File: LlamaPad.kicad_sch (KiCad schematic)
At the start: 0 parts

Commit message: feat: finish schematic rev1
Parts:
- added A1: RaspberryPi_Pico, Module:RaspberryPi_Pico_Common_Unspecified, symbol MCU_Module:RaspberryPi_Pico
- added D1, D10, D11, D12, D13, D14, D15, D16, D17, D18, D2, D3, D4, D5, D6, D7, D8, D9: D, Diode_THT:D_DO-35_SOD27_P7.62mm_Horizontal, symbol Device:D
- added D19, D20, D21, D22, D23, D24, D25, D26, D27, D28, D29, D30, D31, D32, D33, D34: SK6812MINI-E, HackPad:SK6812MINI-E_fixed, symbol SK6812MINI-E:SK6812MINI-E
- added J1: Conn_01x04_Pin, Connector_PinHeader_1.27mm:PinHeader_1x04_P1.27mm_Vertical, symbol Connector:Conn_01x04_Pin
- added REC_A1, REC_B1: RotaryEncoder_Switch, HackPad:RotaryEncoder_Alps_EC11E-Switch_Vertical_H20mm, symbol Device:RotaryEncoder_Switch
- added SW1, SW10, SW11, SW12, SW13, SW14, SW15, SW16, SW2, SW3, SW4, SW5, SW6, SW7, SW8, SW9: SW_Push, Button_Switch_Keyboard:SW_Cherry_MX_1.00u_PCB, symbol Switch:SW_Push
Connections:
- new net: D9.2 (A), SW9.2
- new net: D21.2 (DOUT), D25.4 (DIN)
- new net: D21.4 (DIN), D32.2 (DOUT)
- new net: D15.2 (A), SW14.2
- new net: D4.2 (A), SW4.2
- new net: D30.2 (DOUT), D34.4 (DIN)
- new net: D19.2 (DOUT), D23.4 (DIN)
- new net: D28.2 (DOUT), D32.4 (DIN)
- new net: D26.2 (DOUT), D30.4 (DIN)
- new net: D22.2 (DOUT), D26.4 (DIN)
- new net: D12.2 (A), SW12.2
- new net: D14.2 (A), SW15.2
- new net: D8.2 (A), SW8.2
- new net: D27.2 (DOUT), D31.4 (DIN)
- new net: D23.2 (DOUT), D27.4 (DIN)
- new net: D24.2 (DOUT), D28.4 (DIN)
- new net: D22.4 (DIN), D33.2 (DOUT)
- new net: D10.2 (A), SW10.2
- new net: D29.2 (DOUT), D33.4 (DIN)
- new net: D1.2 (A), SW1.2
- new net: D6.2 (A), SW6.2
- new net: D5.2 (A), SW5.2
- new net: D20.2 (DOUT), D24.4 (DIN)
- new net: D25.2 (DOUT), D29.4 (DIN)
- new net: D11.2 (A), SW11.2
- new net: D20.4 (DIN), D31.2 (DOUT)
- new net: D7.2 (A), SW7.2
- new net: D3.2 (A), SW3.2
- new net: D16.2 (A), SW13.2
- new net: D2.2 (A), SW2.2
- new net: D13.2 (A), SW16.2
- new net ARGB_DATA: A1.17 (GPIO13), D19.4 (DIN)
- new net COL0: A1.6 (GPIO4), SW1.1, SW2.1, SW3.1, SW4.1
- new net COL1: A1.7 (GPIO5), SW5.1, SW6.1, SW7.1, SW8.1
- new net COL2: A1.9 (GPIO6), SW10.1, SW11.1, SW12.1, SW9.1
- new net COL3: A1.10 (GPIO7), SW13.1, SW14.1, SW15.1, SW16.1
- new net COL4: A1.11 (GPIO8), REC_A1.S2, REC_B1.S2
- new net GND: A1.13 (GND), A1.18 (GND), A1.23 (GND), A1.28 (GND), A1.3 (GND), A1.38 (GND), A1.8 (GND), D19.3 (VSS), D20.3 (VSS), D21.3 (VSS), D22.3 (VSS), D23.3 (VSS), D24.3 (VSS), D25.3 (VSS), D26.3 (VSS), D27.3 (VSS), D28.3 (VSS), D29.3 (VSS), D30.3 (VSS), D31.3 (VSS), D32.3 (VSS), D33.3 (VSS), D34.3 (VSS), J1.4 (Pin_4), REC_A1.C, REC_B1.C
- new net OLED_SCL: A1.20 (GPIO15), J1.2 (Pin_2)
- new net OLED_SDA: A1.19 (GPIO14), J1.1 (Pin_1)
- new net REC_A1: A1.12 (GPIO9), REC_A1.B
- new net REC_A2: A1.14 (GPIO10), REC_A1.A
- new net REC_B1: A1.15 (GPIO11), REC_B1.B
- new net REC_B2: A1.16 (GPIO12), REC_B1.A
- new net REC_SW_A2: D18.2 (A), REC_A1.S1
- new net REC_SW_B2: D17.2 (A), REC_B1.S1
- new net ROW0: A1.1 (GPIO0), D1.1 (K), D16.1 (K), D17.1 (K), D5.1 (K), D9.1 (K)
- new net ROW1: A1.2 (GPIO1), D10.1 (K), D15.1 (K), D18.1 (K), D2.1 (K), D6.1 (K)
- new net ROW2: A1.4 (GPIO2), D11.1 (K), D14.1 (K), D3.1 (K), D7.1 (K)
- new net ROW3: A1.5 (GPIO3), D12.1 (K), D13.1 (K), D4.1 (K), D8.1 (K)
- new net VCC: A1.40 (VBUS), D19.1 (VDD), D20.1 (VDD), D21.1 (VDD), D22.1 (VDD), D23.1 (VDD), D24.1 (VDD), D25.1 (VDD), D26.1 (VDD), D27.1 (VDD), D28.1 (VDD), D29.1 (VDD), D30.1 (VDD), D31.1 (VDD), D32.1 (VDD), D33.1 (VDD), D34.1 (VDD), J1.3 (Pin_3)
- no-connect marks 0 -> 17
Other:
- note added: "OLED DISPLAY"
- note added: "PICO"
- note added: "ROTARY ENCODER"
- note added: "SWITCH ARGB"
- note added: "SWITCH MATRIX"

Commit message: feat: PCB rev1 (no traces)
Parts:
- J1: footprint Connector_PinHeader_1.27mm:PinHeader_1x04_P1.27mm_Vertical -> Connector_PinHeader_2.54mm:PinHeader_1x04_P2.54mm_Vertical
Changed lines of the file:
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@@
 			)
 		)
-		(property "Footprint" "Connector_PinHeader_1.27mm:PinHeader_1x04_P1.27mm_Vertical"
+		(property "Footprint" "Connector_PinHeader_2.54mm:PinHeader_1x04_P2.54mm_Vertical"
 			(at 229.87 130.81 0)
 			(effects

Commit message: feat: footprint stuff
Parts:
- SW1, SW10, SW11, SW12, SW13, SW14, SW15, SW16, SW2, SW3, SW4, SW5, SW6, SW7, SW8, SW9: footprint Button_Switch_Keyboard:SW_Cherry_MX_1.00u_PCB -> MX_Hotswap:MX-Hotswap-1U
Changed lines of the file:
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@@
 			)
 		)
-		(property "Footprint" "Button_Switch_Keyboard:SW_Cherry_MX_1.00u_PCB"
+		(property "Footprint" "MX_Hotswap:MX-Hotswap-1U"
 			(at 95.25 57.15 0)
 			(effects
@@
 			)
 		)
-		(property "Footprint" "Button_Switch_Keyboard:SW_Cherry_MX_1.00u_PCB"
+		(property "Footprint" "MX_Hotswap:MX-Hotswap-1U"
 			(at 95.25 69.85 0)
 			(effects
@@
 			)
 		)
-		(property "Footprint" "Button_Switch_Keyboard:SW_Cherry_MX_1.00u_PCB"
+		(property "Footprint" "MX_Hotswap:MX-Hotswap-1U"
 			(at 59.69 82.55 0)
 			(effects
@@
 			)
 		)
-		(property "Footprint" "Button_Switch_Keyboard:SW_Cherry_MX_1.00u_PCB"
+		(property "Footprint" "MX_Hotswap:MX-Hotswap-1U"
 			(at 41.91 44.45 0)
 			(effects
@@
 			)
 		)
-		(property "Footprint" "Button_Switch_Keyboard:SW_Cherry_MX_1.00u_PCB"
+		(property "Footprint" "MX_Hotswap:MX-Hotswap-1U"
 			(at 59.69 57.15 0)
 			(effects
@@
 			)
 		)
-		(property "Footprint" "Button_Switch_Keyboard:SW_Cherry_MX_1.00u_PCB"
+		(property "Footprint" "MX_Hotswap:MX-Hotswap-1U"
 			(at 59.69 44.45 0)
 			(effects
@@
 			)
 		)
-		(property "Footprint" "Button_Switch_Keyboard:SW_Cherry_MX_1.00u_PCB"
+		(property "Footprint" "MX_Hotswap:MX-Hotswap-1U"
 			(at 77.47 69.85 0)
 			(effects
@@
 			)
 		)
-		(property "Footprint" "Button_Switch_Keyboard:SW_Cherry_MX_1.00u_PCB"
+		(property "Footprint" "MX_Hotswap:MX-Hotswap-1U"
 			(at 77.47 82.55 0)
 			(effects
@@
 			)
 		)
-		(property "Footprint" "Button_Switch_Keyboard:SW_Cherry_MX_1.00u_PCB"
+		(property "Footprint" "MX_Hotswap:MX-Hotswap-1U"
 			(at 41.91 82.55 0)
 			(effects
@@
 			)
 		)
-		(property "Footprint" "Button_Switch_Keyboard:SW_Cherry_MX_1.00u_PCB"
+		(property "Footprint" "MX_Hotswap:MX-Hotswap-1U"
 			(at 77.47 57.15 0)
 			(effects
@@
 			)
 		)
-		(property "Footprint" "Button_Switch_Keyboard:SW_Cherry_MX_1.00u_PCB"
+		(property "Footprint" "MX_Hotswap:MX-Hotswap-1U"
 			(at 41.91 57.15 0)
 			(effects
@@
 			)
 		)
-		(property "Footprint" "Button_Switch_Keyboard:SW_Cherry_MX_1.00u_PCB"
+		(property "Footprint" "MX_Hotswap:MX-Hotswap-1U"
 			(at 59.69 69.85 0)
 			(effects
@@
 			)
 		)
-		(property "Footprint" "Button_Switch_Keyboard:SW_Cherry_MX_1.00u_PCB"
+		(property "Footprint" "MX_Hotswap:MX-Hotswap-1U"
 			(at 77.47 44.45 0)
 			(effects
@@
 			)
 		)
-		(property "Footprint" "Button_Switch_Keyboard:SW_Cherry_MX_1.00u_PCB"
+		(property "Footprint" "MX_Hotswap:MX-Hotswap-1U"
 			(at 41.91 69.85 0)
 			(effects
@@
 			)
 		)
-		(property "Footprint" "Button_Switch_Keyboard:SW_Cherry_MX_1.00u_PCB"
+		(property "Footprint" "MX_Hotswap:MX-Hotswap-1U"
 			(at 95.25 82.55 0)
 			(effects
@@
 			)
 		)
-		(property "Footprint" "Button_Switch_Keyboard:SW_Cherry_MX_1.00u_PCB"
+		(property "Footprint" "MX_Hotswap:MX-Hotswap-1U"
 			(at 95.25 44.45 0)
 			(effects

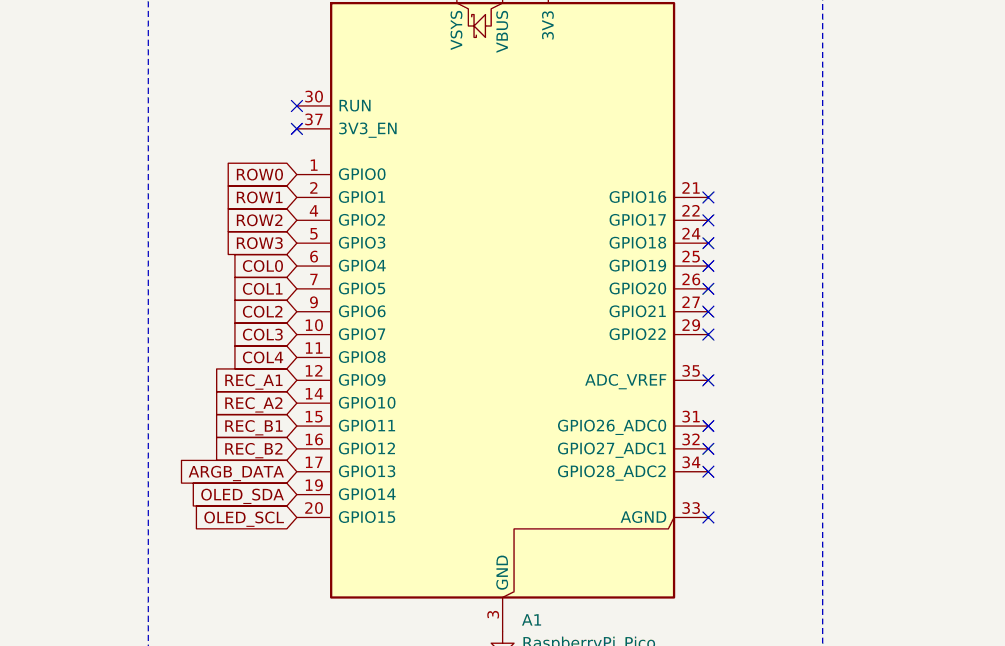
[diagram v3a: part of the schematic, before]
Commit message: feat: route the pcb and change schematic to be easier
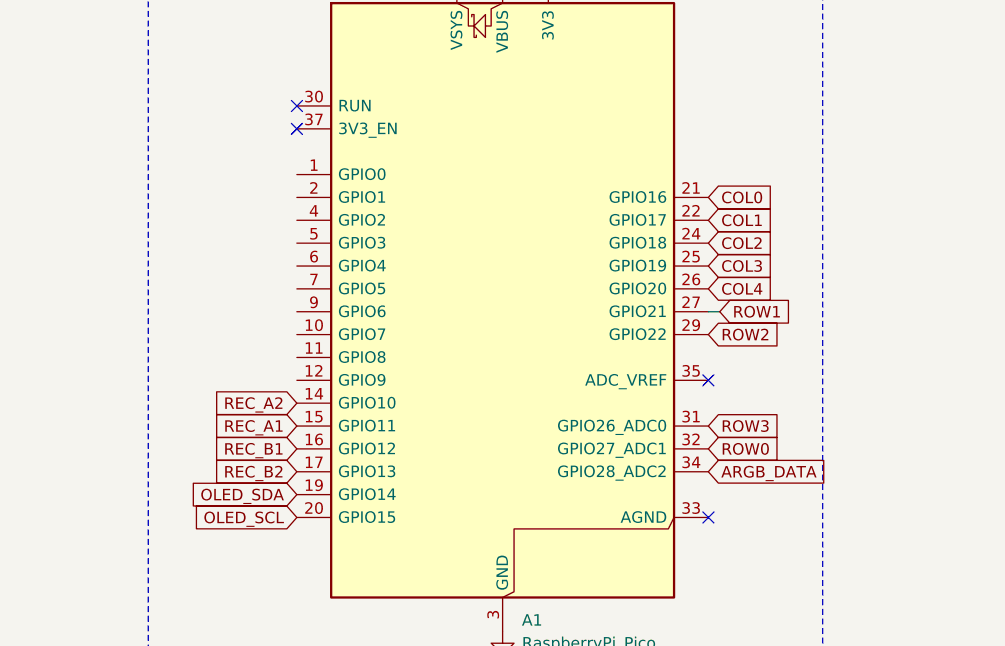
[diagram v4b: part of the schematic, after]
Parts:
- D19, D20, D21, D22, D23, D24, D25, D26, D27, D28, D29, D30, D31, D32, D33, D34: footprint HackPad:SK6812MINI-E_fixed -> Llama_Other:SK6812MINI-E_fixed
- REC_A1, REC_B1: footprint HackPad:RotaryEncoder_Alps_EC11E-Switch_Vertical_H20mm -> RotaryEncoder:RotaryEncoder_Alps_EC11E-Switch_Vertical_H20mm
- SW1, SW10, SW11, SW12, SW13, SW14, SW15, SW16, SW2, SW3, SW4, SW5, SW6, SW7, SW8, SW9: footprint MX_Hotswap:MX-Hotswap-1U -> Switch_MX_Hotswap:MX-Hotswap-1U
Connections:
- net ARGB_DATA: now also A1.34 (GPIO28_ADC2); no longer A1.17 (GPIO13)
- net COL0: now also A1.21 (GPIO16); no longer A1.6 (GPIO4)
- net COL1: now also A1.22 (GPIO17); no longer A1.7 (GPIO5)
- net COL2: now also A1.24 (GPIO18); no longer A1.9 (GPIO6)
- net COL3: now also A1.25 (GPIO19); no longer A1.10 (GPIO7)
- net COL4: now also A1.26 (GPIO20); no longer A1.11 (GPIO8)
- net REC_A1: now also A1.15 (GPIO11); no longer A1.12 (GPIO9)
- net REC_B1: now also A1.16 (GPIO12); no longer A1.15 (GPIO11)
- net REC_B2: now also A1.17 (GPIO13); no longer A1.16 (GPIO12)
- net ROW0: now also A1.32 (GPIO27_ADC1); no longer A1.1 (GPIO0)
- net ROW1: now also A1.27 (GPIO21); no longer A1.2 (GPIO1)
- net ROW2: now also A1.29 (GPIO22); no longer A1.4 (GPIO2)
- net ROW3: now also A1.31 (GPIO26_ADC0); no longer A1.5 (GPIO3)
- no-connect marks 17 -> 7
